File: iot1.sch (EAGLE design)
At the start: 32 parts, among them IC1 MEGA8-P, IC2 7805T, J1 DCJ0202, U2 HTU21D, X1 22-23-2041, X2 A1944-50

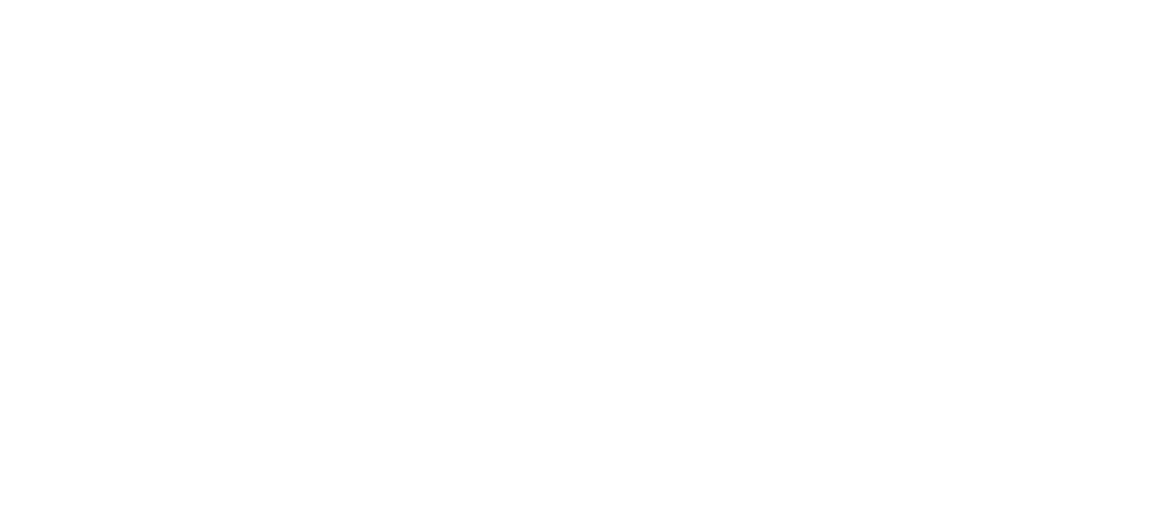
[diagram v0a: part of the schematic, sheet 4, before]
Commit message: adc
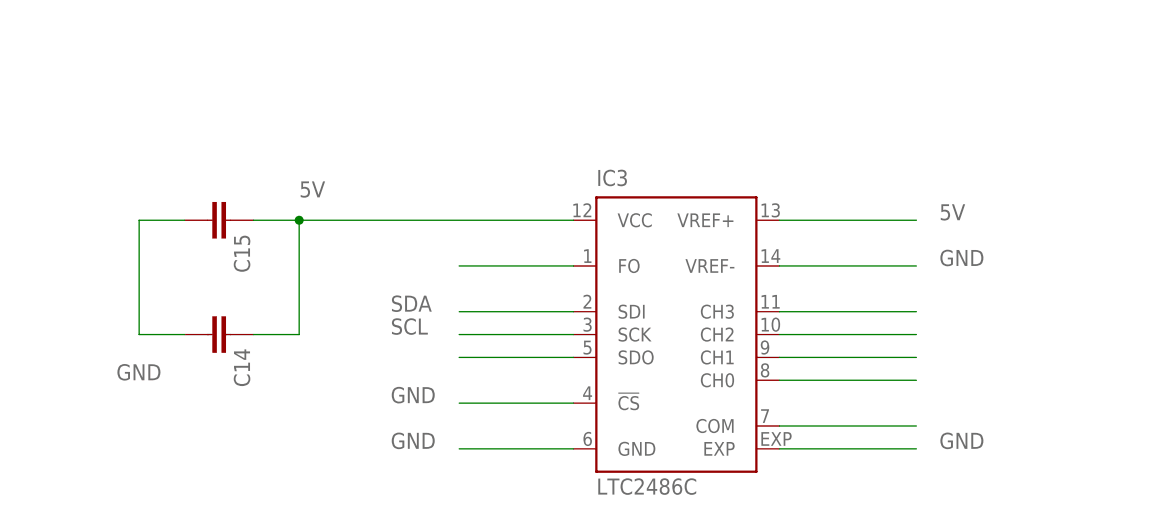
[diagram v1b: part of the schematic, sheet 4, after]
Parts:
- added C14, C15: (no value), rcl:C-EUC0603
- added IC3: LTC2486C, linear-technology:LTC2486C
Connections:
- removed net N$29: IC1.PC4(ADC4/SDA)
- new net N$71: IC3.CH3
- new net N$74: IC3.CH2
- new net N$75: IC3.CH1
- new net N$76: IC3.CH0
- new net N$77: IC3.COM
- net 5V: now also C14.1, C15.1, IC3.VCC, IC3.VREF+
- net GND: now also C14.2, C15.2, IC3.!CS, IC3.EXP, IC3.GND, IC3.VREF-
- net N$31: now also IC3.SDO; no longer IC1.PC5(ADC5/SCL)
- net SCL: now also IC1.PC5(ADC5/SCL), IC3.FO, IC3.SCK
- net SDA: now also IC1.PC4(ADC4/SDA), IC3.SDI
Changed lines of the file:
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@@
 <part name="S1" library="switch-omron" library_urn="urn:adsk.eagle:library:377" deviceset="10-XX" device="" package3d_urn="urn:adsk.eagle:package:27496/1"/>
 <part name="C13" library="rcl" library_urn="urn:adsk.eagle:library:334" deviceset="C-EU" device="050-025X075" package3d_urn="urn:adsk.eagle:package:23637/1" value="0.1u"/>
+<part name="IC3" library="linear-technology" library_urn="urn:adsk.eagle:library:261" deviceset="LTC2486" device="" package3d_urn="urn:adsk.eagle:package:16069/1" technology="C"/>
+<part name="C14" library="rcl" library_urn="urn:adsk.eagle:library:334" deviceset="C-EU" device="C0603" package3d_urn="urn:adsk.eagle:package:23616/2"/>
+<part name="C15" library="rcl" library_urn="urn:adsk.eagle:library:334" deviceset="C-EU" device="C0603" package3d_urn="urn:adsk.eagle:package:23616/2"/>
 </parts>
 <sheets>
@@
 </segment>
 </net>
-<net name="N$29" class="0">
+<net name="SDA" class="0">
 <segment>
 <pinref part="IC1" gate="G$1" pin="PC4(ADC4/SDA)"/>
 <wire x1="162.56" y1="154.94" x2="187.96" y2="154.94" width="0.1524" layer="91"/>
-</segment>
-</net>
-<net name="N$31" class="0">
+<label x="190.5" y="154.94" size="1.778" layer="95"/>
+</segment>
+</net>
+<net name="SCL" class="0">
 <segment>
 <pinref part="IC1" gate="G$1" pin="PC5(ADC5/SCL)"/>
 <wire x1="162.56" y1="152.4" x2="187.96" y2="152.4" width="0.1524" layer="91"/>
+<label x="190.5" y="152.4" size="1.778" layer="95"/>
 </segment>
 </net>
@@
 <attribute name="NAME" x="69.723" y="135.1026" size="1.778" layer="95"/>
 <attribute name="VALUE" x="69.723" y="130.0226" size="1.778" layer="96"/>
+</instance>
+<instance part="IC3" gate="G$1" x="81.28" y="76.2" smashed="yes">
+<attribute name="NAME" x="73.66" y="92.71" size="1.778" layer="95"/>
+<attribute name="VALUE" x="73.66" y="58.42" size="1.778" layer="96"/>
+</instance>
+<instance part="C14" gate="G$1" x="33.02" y="76.2" smashed="yes" rot="R270">
+<attribute name="NAME" x="33.401" y="74.676" size="1.778" layer="95" rot="R270"/>
+<attribute name="VALUE" x="28.321" y="74.676" size="1.778" layer="96" rot="R270"/>
+</instance>
+<instance part="C15" gate="G$1" x="33.02" y="88.9" smashed="yes" rot="R270">
+<attribute name="NAME" x="33.401" y="87.376" size="1.778" layer="95" rot="R270"/>
+<attribute name="VALUE" x="28.321" y="87.376" size="1.778" layer="96" rot="R270"/>
 </instance>
 </instances>
@@
 <junction x="25.4" y="137.16"/>
 </segment>
+<segment>
+<pinref part="C15" gate="G$1" pin="2"/>
+<wire x1="27.94" y1="88.9" x2="22.86" y2="88.9" width="0.1524" layer="91"/>
+<pinref part="C14" gate="G$1" pin="2"/>
+<wire x1="22.86" y1="88.9" x2="22.86" y2="76.2" width="0.1524" layer="91"/>
+<wire x1="22.86" y1="76.2" x2="27.94" y2="76.2" width="0.1524" layer="91"/>
+<label x="20.32" y="71.12" size="1.778" layer="95"/>
+</segment>
+<segment>
+<pinref part="IC3" gate="G$1" pin="GND"/>
+<wire x1="71.12" y1="63.5" x2="58.42" y2="63.5" width="0.1524" layer="91"/>
+<label x="50.8" y="63.5" size="1.778" layer="95"/>
+</segment>
+<segment>
+<pinref part="IC3" gate="G$1" pin="!CS"/>
+<wire x1="71.12" y1="68.58" x2="58.42" y2="68.58" width="0.1524" layer="91"/>
+<label x="50.8" y="68.58" size="1.778" layer="95"/>
+</segment>
+<segment>
+<pinref part="IC3" gate="G$1" pin="VREF-"/>
+<wire x1="93.98" y1="83.82" x2="109.22" y2="83.82" width="0.1524" layer="91"/>
+<label x="111.76" y="83.82" size="1.778" layer="95"/>
+</segment>
+<segment>
+<pinref part="IC3" gate="G$1" pin="EXP"/>
+<wire x1="93.98" y1="63.5" x2="109.22" y2="63.5" width="0.1524" layer="91"/>
+<label x="111.76" y="63.5" size="1.778" layer="95"/>
+</segment>
 </net>
 <net name="SOIL_MOISTURE_1" class="0">
@@
 <wire x1="68.58" y1="142.24" x2="68.58" y2="137.16" width="0.1524" layer="91"/>
 </segment>
-</net>
+<segment>
+<pinref part="C14" gate="G$1" pin="1"/>
+<wire x1="35.56" y1="76.2" x2="40.64" y2="76.2" width="0.1524" layer="91"/>
+<pinref part="C15" gate="G$1" pin="1"/>
+<wire x1="35.56" y1="88.9" x2="40.64" y2="88.9" width="0.1524" layer="91"/>
+<wire x1="40.64" y1="88.9" x2="40.64" y2="76.2" width="0.1524" layer="91"/>
+<label x="40.64" y="91.44" size="1.778" layer="95"/>
+<pinref part="IC3" gate="G$1" pin="VCC"/>
+<wire x1="71.12" y1="88.9" x2="40.64" y2="88.9" width="0.1524" layer="91"/>
+<junction x="40.64" y="88.9"/>
+</segment>
+<segment>
+<pinref part="IC3" gate="G$1" pin="VREF+"/>
+<wire x1="93.98" y1="88.9" x2="109.22" y2="88.9" width="0.1524" layer="91"/>
+<label x="111.76" y="88.9" size="1.778" layer="95"/>
+</segment>
+</net>
+<net name="SDA" class="0">
+<segment>
+<pinref part="IC3" gate="G$1" pin="SDI"/>
+<wire x1="71.12" y1="78.74" x2="58.42" y2="78.74" width="0.1524" layer="91"/>
+<label x="50.8" y="78.74" size="1.778" layer="95"/>
+</segment>
+</net>
+<net name="N$31" class="0">
+<segment>
+<pinref part="IC3" gate="G$1" pin="SDO"/>
+<wire x1="71.12" y1="73.66" x2="58.42" y2="73.66" width="0.1524" layer="91"/>
+</segment>
+</net>
+<net name="N$71" class="0">
+<segment>
+<pinref part="IC3" gate="G$1" pin="CH3"/>
+<wire x1="93.98" y1="78.74" x2="109.22" y2="78.74" width="0.1524" layer="91"/>
+</segment>
+</net>
+<net name="N$74" class="0">
+<segment>
+<pinref part="IC3" gate="G$1" pin="CH2"/>
+<wire x1="93.98" y1="76.2" x2="109.22" y2="76.2" width="0.1524" layer="91"/>
+</segment>
+</net>
+<net name="N$75" class="0">
+<segment>
+<pinref part="IC3" gate="G$1" pin="CH1"/>
+<wire x1="93.98" y1="73.66" x2="109.22" y2="73.66" width="0.1524" layer="91"/>
+</segment>
+</net>
+<net name="N$76" class="0">
+<segment>
+<pinref part="IC3" gate="G$1" pin="CH0"/>
+<wire x1="93.98" y1="71.12" x2="109.22" y2="71.12" width="0.1524" layer="91"/>
+</segment>
+</net>
+<net name="N$77" class="0">
+<segment>
+<pinref part="IC3" gate="G$1" pin="COM"/>
+<wire x1="93.98" y1="66.04" x2="109.22" y2="66.04" width="0.1524" layer="91"/>
+</segment>
+</net>
+<net name="SCL" class="0">
+<segment>
+<pinref part="IC3" gate="G$1" pin="FO"/>
+<wire x1="71.12" y1="83.82" x2="58.42" y2="83.82" width="0.1524" layer="91"/>
+</segment>
+<segment>
+<pinref part="IC3" gate="G$1" pin="SCK"/>
+<wire x1="71.12" y1="76.2" x2="58.42" y2="76.2" width="0.1524" layer="91"/>
+<label x="50.8" y="76.2" size="1.778" layer="95"/>
+</segment>
+</net>
